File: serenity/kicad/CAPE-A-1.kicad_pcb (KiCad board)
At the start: 4 copper layers, 55 x 35 mm, 31 parts

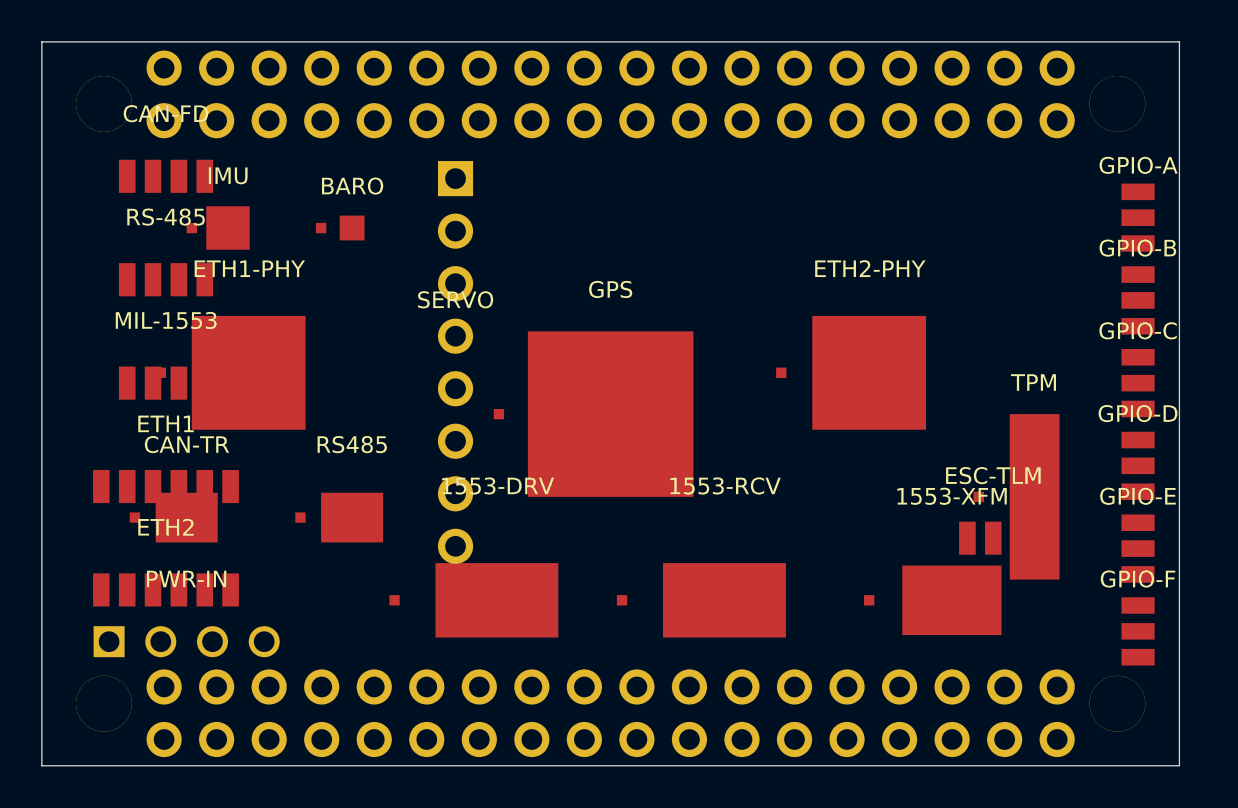
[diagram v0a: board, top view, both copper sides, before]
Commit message: cape fixes
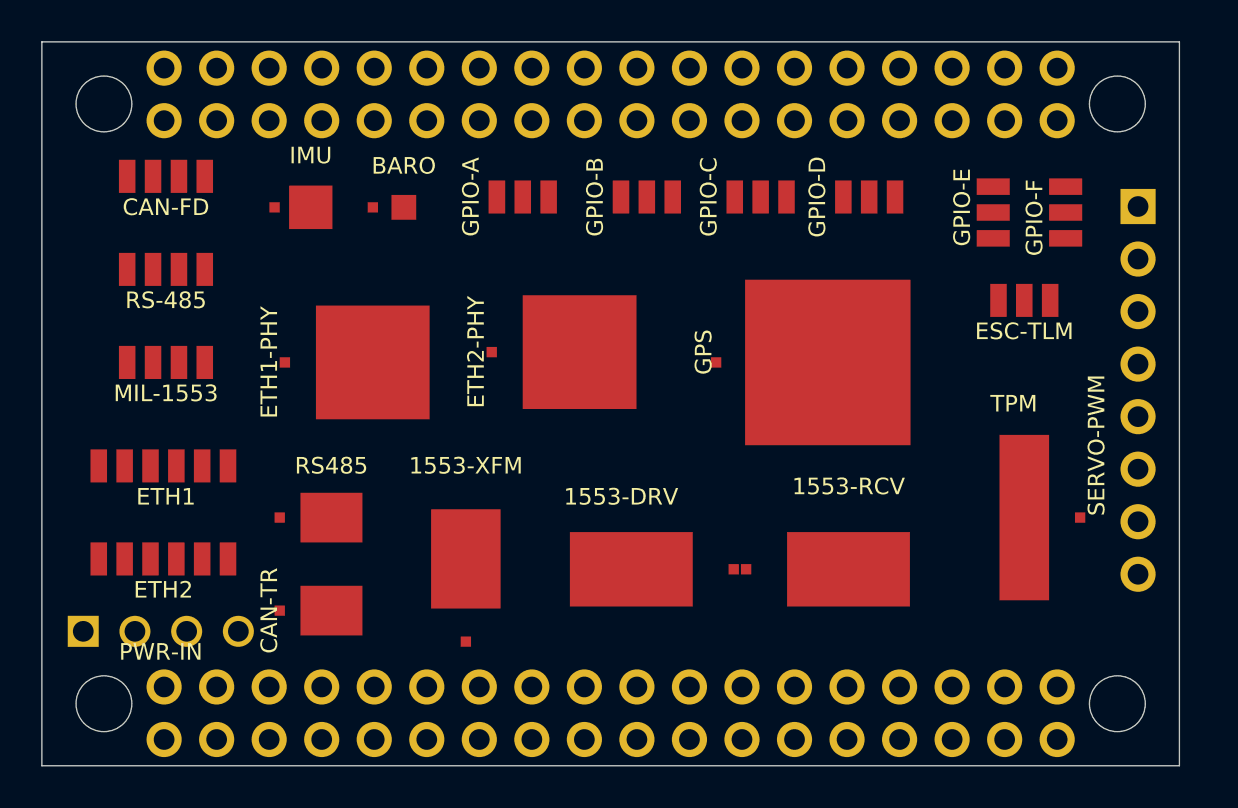
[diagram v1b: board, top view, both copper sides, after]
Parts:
- removed SERVO: 1x8-SERVO-PWM, Connector_PinHeader_2.54mm
- added SERVO-PWM: 1x8-SERVO-PWM, Connector_PinHeader_2.54mm, F.Cu at (174.0, 104.3)
- moved GPIO-A 29.8 mm to (144.2, 95.0), turned to 90 degrees
- moved GPIO-B 24.3 mm to (150.2, 95.0), turned to 90 degrees
- moved 1553-XFM 23.6 mm to (141.5, 112.5), turned to 90 degrees
- moved GPIO-F 20.6 mm to (170.5, 95.8)
- moved GPIO-C 20.3 mm to (155.8, 95.0), turned to 90 degrees
- moved GPIO-D 18.4 mm to (161.0, 95.0), turned to 90 degrees
- moved GPIO-E 17.7 mm to (167.0, 95.8)
- moved ETH2-PHY 14.0 mm to (147.0, 102.5)
- moved ESC-TLM 11.6 mm to (168.5, 100.0)
- moved GPS 10.8 mm to (159.0, 103.0)
- moved CAN-TR 8.32 mm to (135.0, 115.0)
- moved 1553-DRV 6.67 mm to (149.5, 113.0), turned to 180 degrees
- moved 1553-RCV 6.18 mm to (160.0, 113.0)
- moved ETH1-PHY 6.02 mm to (137.0, 103.0)
- moved IMU 4.12 mm to (134.0, 95.5)
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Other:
- board text added: "UAV Resillient Control Cape For the PocketBeagle2 CC BY 4.0 — May 2026 Steve Griffing PE(CSE), CISSP-ISSEP, CPP Griffing Technology LLC www.github.com/Stab-Rabbit-Coding"
- board text removed: "CC BY 4.0 — Stab-Rabbit-Coding"
- board text removed: "Serenity UAV — FC Cape Rev M"
